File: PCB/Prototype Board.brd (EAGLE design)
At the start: 55.9 x 76.2 mm, 78 parts, among them Q1 S8050, Q10 20V/0.2A/8MHz/1.2Ω/1Vth, Q2 20V/0.2A/8MHz/1.2Ω/1Vth, Q3 20V/4.2A/52mΩ/1.4W, Q4 S8050, Q5 20V/0.2A/8MHz/1.2Ω/1Vth, Q6 20V/0.2A/8MHz/1.2Ω/1Vth, Q7 20V/0.2A/8MHz/1.2Ω/1Vth, Q8 20V/0.2A/8MHz/1.2Ω/1Vth, U1 9DoF IMU, U2 MCP73831, U3 ESP-WROOM-32, U5 DWM1000

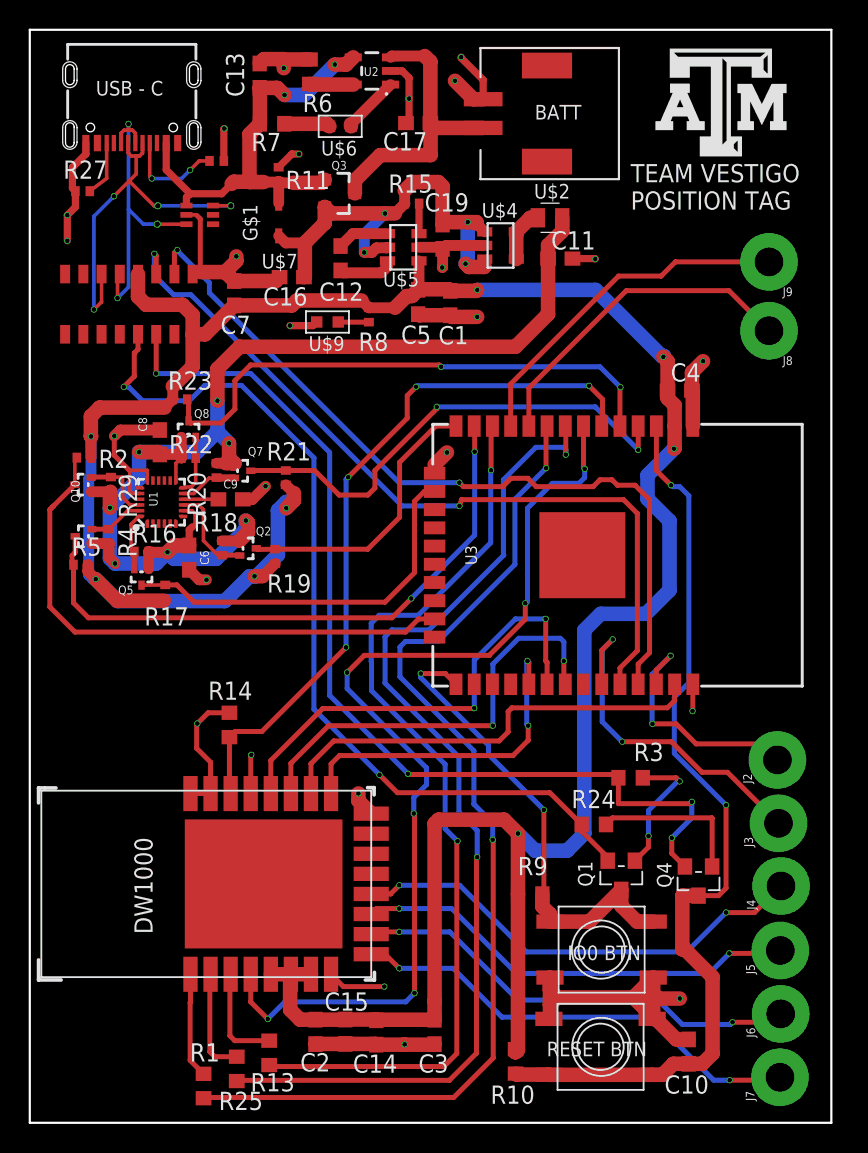
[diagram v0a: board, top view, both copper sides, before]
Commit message: Finalized PCB
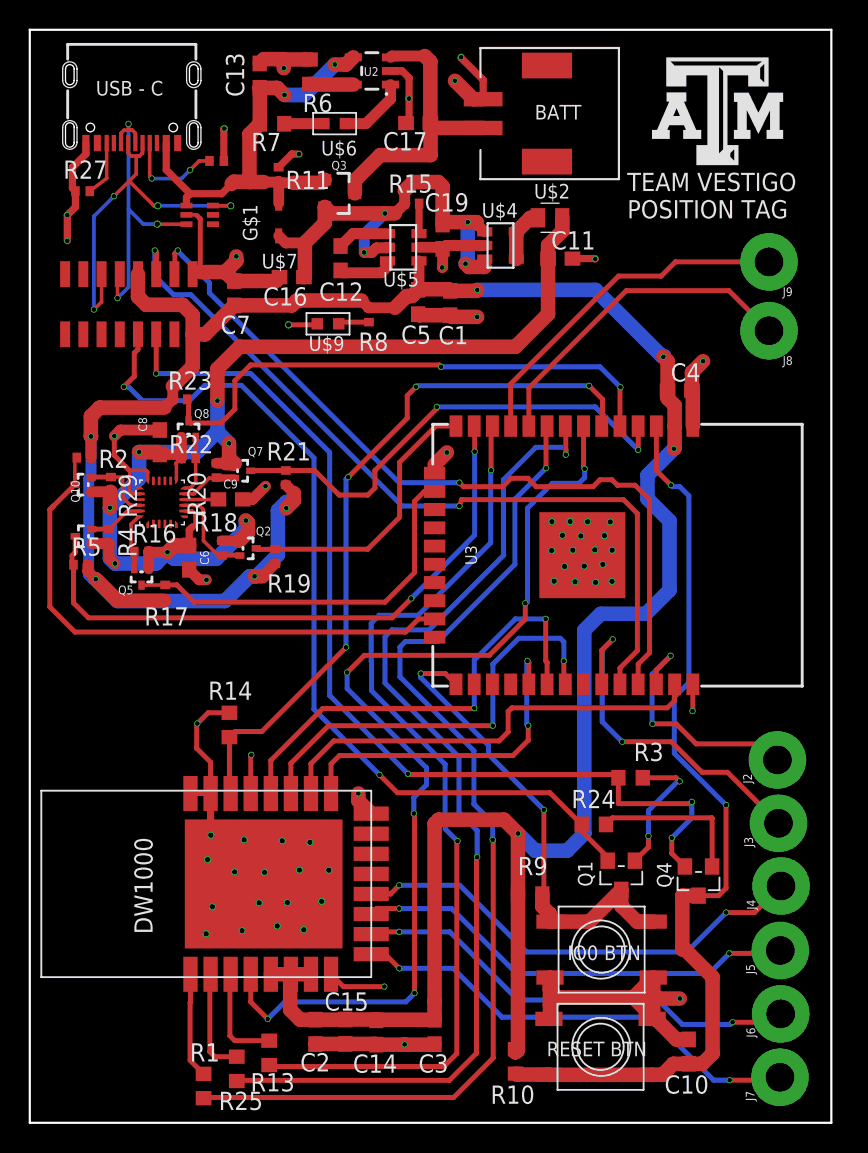
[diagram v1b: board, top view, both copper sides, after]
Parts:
- removed U1: 9DoF IMU, SparkFun-Sensors:QFN24-3X3
- added U$12: ICM20948, customlib:ICM20948
- moved U$6 0.43 mm to (21.3, 69.7), turned to 180 degrees
- moved U$9 0.13 mm to (20.8, 55.7), turned to 0 degrees
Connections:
- net 1.8V: now also U$12.13, U$12.8; no longer U1.13, U1.8
- net CHG_LED: now also U$6.2; no longer U$6.1
- net FSYNC/IO36: now also U$12.11; no longer U1.11
- net GND: now also U$12.18, U$12.20, U$9.1, U3.GND; no longer U$9.2, U1.18, U1.20
- net GPIO12/SDO: now also U$12.9; no longer U1.9
- net GPIO13/SDI: now also U$12.24; no longer U1.24
- net GPIO14/SCLK: now also U$12.23; no longer U1.23
- net GPIO15/CS: now also U$12.22; no longer U1.22
- net INT/IO39: now also U$12.12; no longer U1.12
- net N$13: now also U$12.10; no longer U1.10
- net N$4: now also U$9.2; no longer U$9.1
- net N$7: now also U$6.1; no longer U$6.2
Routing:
- net GND: track 126.2 -> 194.7 mm, vias 25 -> 60
- net N$7: track 4.05 -> 4.87 mm
